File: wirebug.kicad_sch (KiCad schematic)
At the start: 1 part

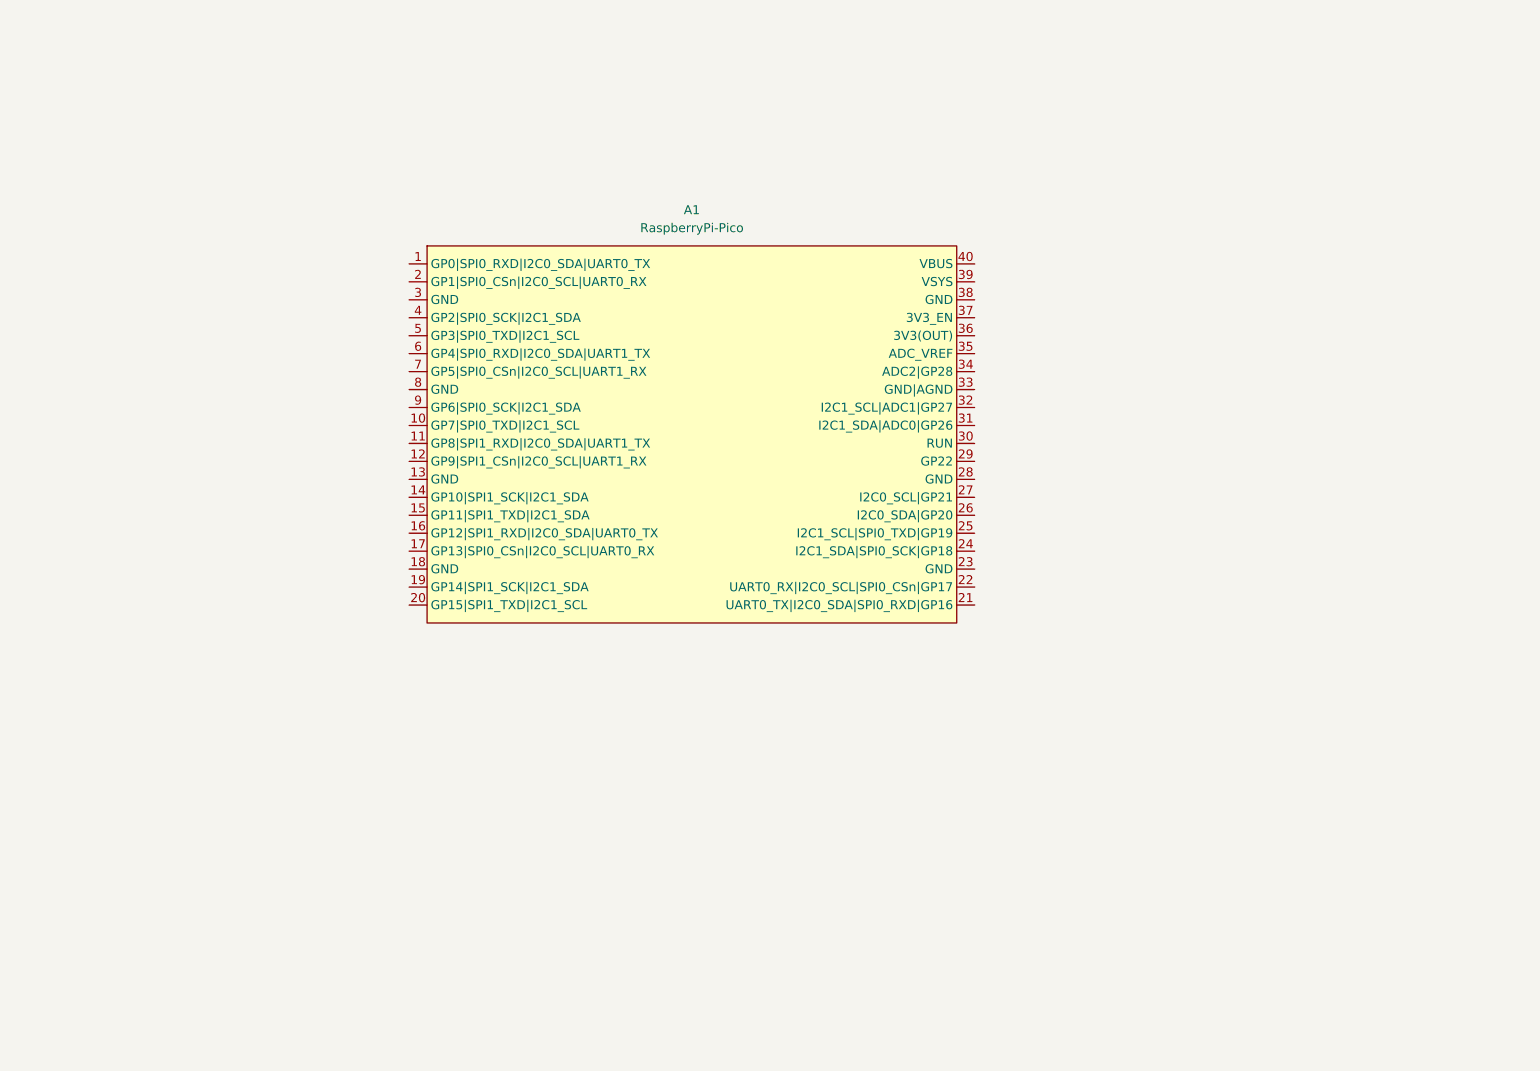
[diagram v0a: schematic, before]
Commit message: First draft
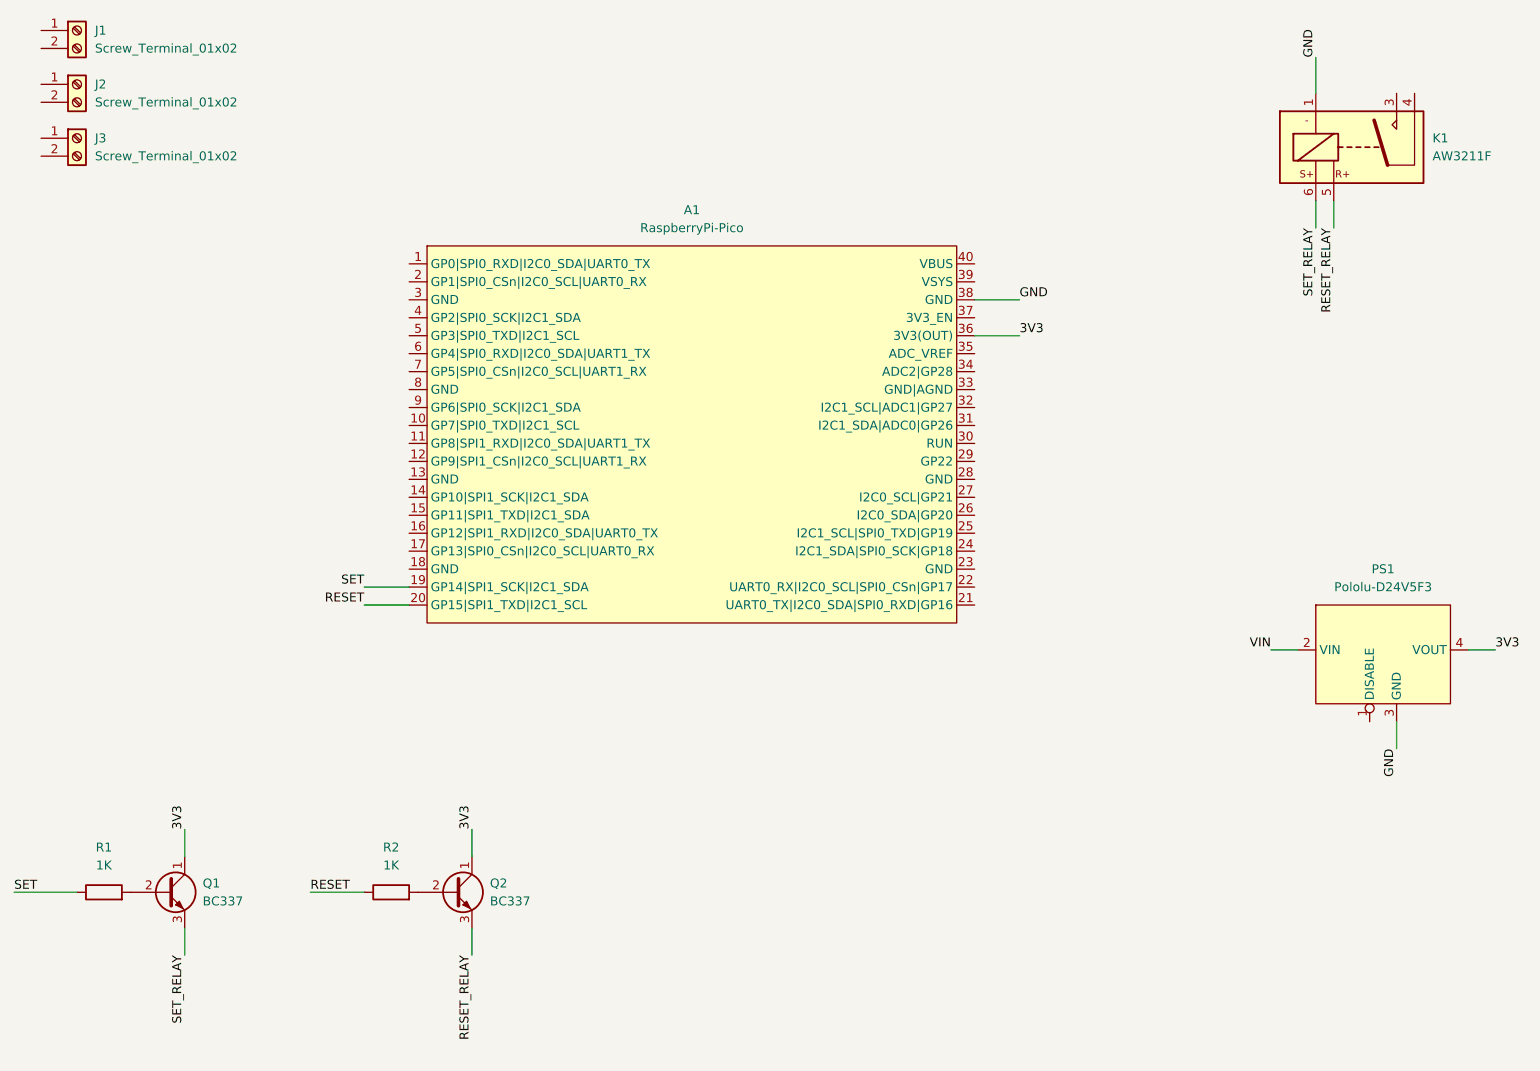
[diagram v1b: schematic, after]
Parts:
- added J1, J2, J3: Screw_Terminal_01x02, TerminalBlock:TerminalBlock_Altech_AK300-2_P5.00mm, symbol Connector:Screw_Terminal_01x02
- added K1: AW3211F, twyleg-misc:Relay_Panasonic_AW3211F_THT, symbol twyleg-misc:AW3211F
- added PS1: Pololu-D24V5F3, twyleg-voltage-regulators:Pololu-D24V5F3-Dev, symbol twyleg-voltage-regulators:Pololu-D24V5F3
- added Q1, Q2: BC337, Package_TO_SOT_THT:TO-92_Inline, symbol Transistor_BJT:BC337
- added R1, R2: 1K, Resistor_THT:R_Axial_DIN0207_L6.3mm_D2.5mm_P7.62mm_Horizontal, symbol Device:R
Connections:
- net SET: now reaches A1.19 (GP14|SPI1_SCK|I2C1_SDA)
- net SET: now also R1.1
- net RESET: now reaches A1.20 (GP15|SPI1_TXD|I2C1_SCL)
- net RESET: now also R2.1
- net 3V3: now reaches A1.36 (3V3(OUT))
- net 3V3: now also PS1.4 (VOUT), Q1.1 (C), Q2.1 (C)
- net GND: now reaches A1.38 (GND)
- net GND: now also K1.1, PS1.3 (GND)
- new net: Q2.2 (B), R2.2
- new net: Q1.2 (B), R1.2
- new net RESET_RELAY: K1.5, Q2.3 (E)
- new net SET_RELAY: K1.6, Q1.3 (E)
- new net VIN: PS1.2 (VIN)
